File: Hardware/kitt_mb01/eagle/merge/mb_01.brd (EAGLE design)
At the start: 160 x 100 mm, 123 parts, among them CON1 ARDUINO_UNO, IC1.01 RT8293A, IC2.00 BQ24266RGET, IC3.01 LSM9DS1, P2 S2B-PH-K-S(LF)(SN), U6.01 TPS61032RSARPSDO-G16, U7.01 SI1922EDH, X7.02 HEAD-LIGHT, X7.03 TAIL-LIGHT, X7.05 MOTOR

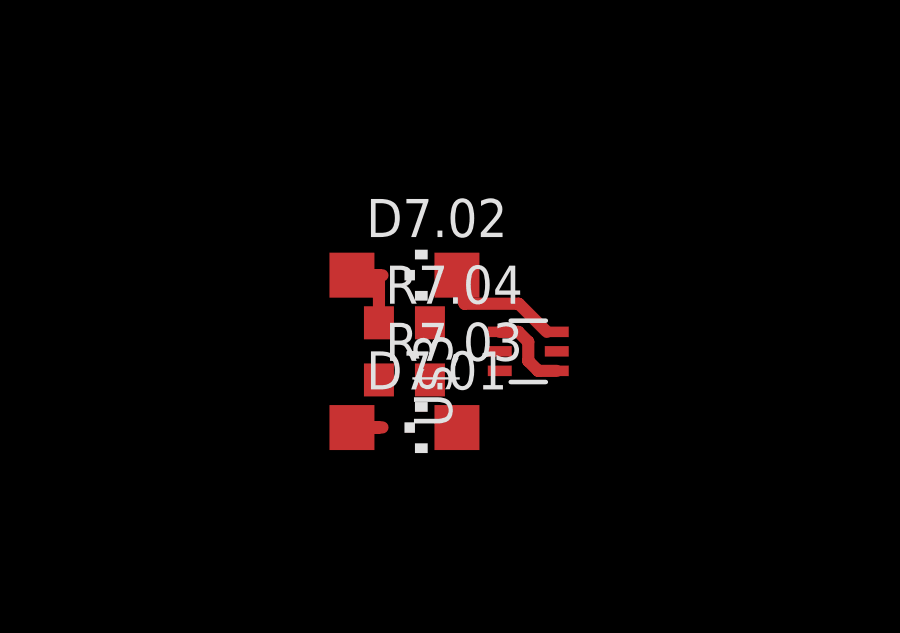
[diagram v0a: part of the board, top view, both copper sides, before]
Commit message: snapshot of board merge
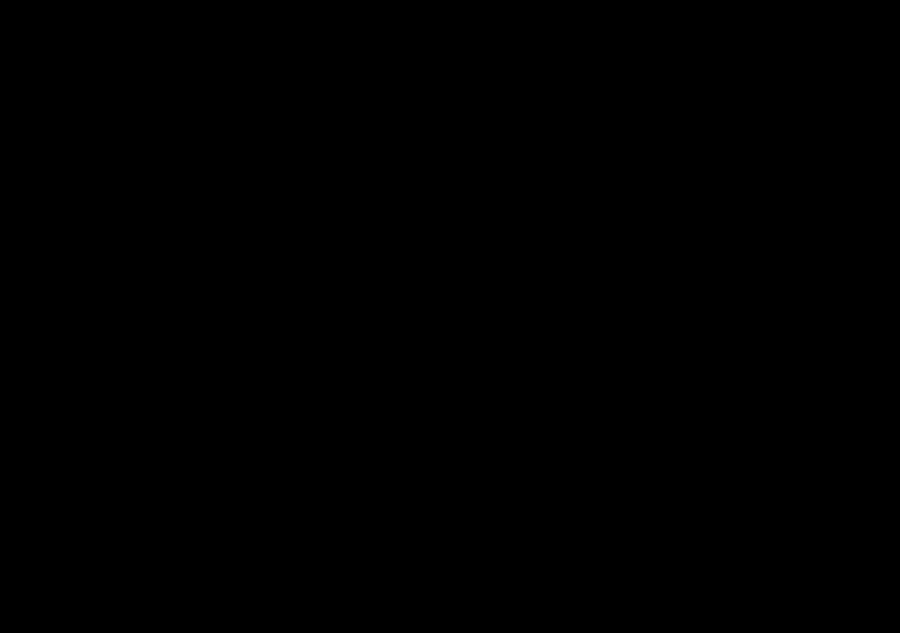
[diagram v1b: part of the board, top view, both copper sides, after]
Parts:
- removed D7.01, D7.02: (no value), led:CHIPLED_1206
- removed R7,03, R7.04: 330R, rcl:R0603
- U$3: value SI1922EDH -> (none); device kitt.ic:SC70-6 -> frames:A4L-LOC
- moved U$3 110.4 mm to (-48.3, -42.5), turned to 0 degrees
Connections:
- removed net N$3: D7.01.C, U$3.6
- removed net N$4: D7.01.A, R7,03.1
- removed net N$5: D7.02.A, R7.04.1
- removed net N$7: D7.02.C, U$3.3
- net +3V3: no longer R7,03.2, R7.04.2
- net GND: no longer U$3.1, U$3.4
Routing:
- net N$7: track 4.12 -> 0.00 mm
- net N$5: track 3.51 -> 0.00 mm
- net GND: track 245.3 -> 242.5 mm
- net N$4: track 1.92 -> 0.00 mm
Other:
- board text added: "D.Hoeginger/A.Gessler"
- board text added: "KITT-MB01 PCB LAYOUT"
- board text added: "Kit for Intelligent and Trainable Trackcars"
- board text removed: "<-- IDK"
- board text removed: "GND@2"
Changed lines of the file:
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@@
 <layers>
 <layer number="1" name="Top" color="4" fill="1" visible="yes" active="yes"/>
-<layer number="2" name="Route2" color="29" fill="0" visible="no" active="yes"/>
+<layer number="2" name="Route2" color="29" fill="0" visible="yes" active="yes"/>
 <layer number="3" name="Route3" color="24" fill="9" visible="yes" active="yes"/>
 <layer number="14" name="Route14" color="1" fill="6" visible="no" active="no"/>
@@
 <wire x1="102.6" y1="73.9" x2="49.1" y2="73.9" width="0.4064" layer="20"/>
 <wire x1="46.7" y1="71.4" x2="46.7" y2="23.1" width="0.4064" layer="20"/>
-<text x="20.16125" y="7.77875" size="1.778" layer="2">GND@2</text>
-<text x="147.32" y="4.60375" size="1.778" layer="2">GND@2</text>
-<text x="143.03375" y="87.78875" size="1.778" layer="2">GND@2</text>
-<text x="8.5725" y="89.8525" size="1.778" layer="2">GND@2</text>
 <text x="48.26" y="64.92875" size="1.9304" layer="25" font="vector">+</text>
 <text x="102.5525" y="35.40125" size="1.016" layer="25" font="vector" rot="R90">SHUNT</text>
@@
 <text x="106.600625" y="46.51375" size="1.778" layer="51">&lt;-- Head Light</text>
 <hole x="101.6" y="27.94" drill="1.6"/>
-<text x="15.5575" y="52.07" size="1.6764" layer="49" rot="R90">&lt;-- IDK</text>
 <text x="20.32" y="37.7825" size="1.6764" layer="49">SPEEDBOARD --&gt;
 LAPDETECTOR --&gt;</text>
@@
 <text x="91.7575" y="8.5725" size="1.778" layer="48">RAILS POURS</text>
 <text x="70.1675" y="6.0325" size="1.778" layer="48">ARDUINO&lt;-&gt;RAILS</text>
+<text x="168.91" y="-22.225" size="1.9304" layer="48" font="vector">D.Hoeginger/A.Gessler</text>
+<text x="114.3" y="-21.9075" size="1.9304" layer="48" font="vector">KITT-MB01 PCB LAYOUT</text>
+<text x="114.3" y="-36.5125" size="1.9304" layer="48" font="vector">Kit for Intelligent and
+Trainable Trackcars</text>
 </plain>
 <attributes>
@@
 <attribute name="MPN" value="" x="102.71125" y="46.51375" size="1.016" layer="27" font="vector" rot="R270" display="off"/>
 </element>
-<element name="D7.01" library="led" package="CHIPLED_1206" value="" x="14.049375" y="43.100625" rot="R270"/>
-<element name="U$3" library="kitt.ic" package="SC70-6" value="SI1922EDH" x="18.176875" y="45.640625" rot="R90"/>
-<element name="R7,03" library="rcl" package="R0603" value="330R" x="14.049375" y="44.688125"/>
-<element name="R7.04" library="rcl" package="R0603" value="330R" x="14.049375" y="46.593125"/>
-<element name="D7.02" library="led" package="CHIPLED_1206" value="" x="14.049375" y="48.180625" rot="R270"/>
 <element name="R0.02" library="rcl" package="R1206" value="SHUNT" x="51.7525" y="56.753125" rot="R270"/>
 <element name="D7.03" library="led" package="CHIPLED_1206" value="" x="101.6" y="54.61" rot="MR90"/>
@@
 <element name="REF1" library="kitt.refs" package="REF_LAYERS" value="REF.LAYERS" x="102.5525" y="67.945" rot="R270"/>
 <element name="REF2" library="kitt.refs" package="REF_LOGO_UASUA" value="REF.LOGO.UASUA" x="77.63" y="65.405" rot="MR270"/>
+<element name="U$3" library="frames" package="A4L-LOC" value="" x="-48.26" y="-42.545"/>
 </elements>
 <signals>
@@
 <wire x1="92.948125" y1="40.9575" x2="94.853125" y2="39.0525" width="1.6764" layer="1"/>
 <wire x1="94.853125" y1="39.0525" x2="100.0125" y2="39.0525" width="1.6764" layer="1"/>
-<contactref element="U$3" pad="1"/>
-<contactref element="U$3" pad="4"/>
-<wire x1="17.226875" y1="46.290625" x2="17.844375" y2="46.290625" width="0.4064" layer="1"/>
-<wire x1="17.844375" y1="46.290625" x2="18.176875" y2="45.958125" width="0.4064" layer="1"/>
-<wire x1="18.176875" y1="45.958125" x2="18.176875" y2="45.323125" width="0.4064" layer="1"/>
-<wire x1="18.176875" y1="45.323125" x2="18.509375" y2="44.990625" width="0.4064" layer="1"/>
-<wire x1="19.126875" y1="44.990625" x2="18.509375" y2="44.990625" width="0.4064" layer="1"/>
 <wire x1="69.8025" y1="41.91" x2="67.945" y2="41.91" width="0.4064" layer="1"/>
 <wire x1="67.945" y1="41.91" x2="66.28" y2="41.91" width="0.4064" layer="1"/>
@@
 <wire x1="103.505" y1="27.785" x2="103.35" y2="27.94" width="0.6096" layer="16"/>
 <wire x1="89.349375" y1="47.550625" x2="88.9" y2="47.3225" width="0" layer="19" extent="1-16"/>
-<wire x1="19.126875" y1="44.990625" x2="48.26" y2="55.331125" width="0" layer="19" extent="1-1"/>
 </signal>
 <signal name="+12V">
@@
 <wire x1="84.29625" y1="43.4975" x2="84.29625" y2="43.244375" width="0.254" layer="1"/>
 <wire x1="84.29625" y1="43.244375" x2="84.61375" y2="43.00625" width="0.254" layer="1"/>
-<contactref element="R7.04" pad="2"/>
-<contactref element="R7,03" pad="2"/>
 <contactref element="R7.01" pad="2"/>
 <contactref element="R7,01" pad="2"/>
@@
 <wire x1="51.865" y1="50.8" x2="54.9275" y2="50.8" width="1.016" layer="1"/>
 <wire x1="76.835" y1="42.148125" x2="77.94625" y2="42.148125" width="0" layer="19" extent="1-3"/>
-<wire x1="14.899375" y1="46.593125" x2="51.865" y2="50.8" width="0" layer="19" extent="1-1"/>
-<wire x1="14.899375" y1="44.688125" x2="14.899375" y2="46.593125" width="0" layer="19" extent="1-1"/>
 </signal>
 <signal name="N$17">
@@
 <wire x1="60.6275" y1="62.70625" x2="58.57875" y2="62.70875" width="0" layer="19" extent="1-1"/>
 </signal>
-<signal name="N$3">
-<contactref element="D7.01" pad="C"/>
-<contactref element="U$3" pad="6"/>
-<wire x1="15.539375" y1="43.100625" x2="15.799375" y2="43.100625" width="0.4064" layer="1"/>
-<wire x1="15.799375" y1="43.100625" x2="17.226875" y2="44.990625" width="0" layer="19" extent="1-1"/>
-</signal>
-<signal name="N$4">
-<contactref element="R7,03" pad="1"/>
-<contactref element="D7.01" pad="A"/>
-<wire x1="13.316875" y1="43.105625" x2="12.299375" y2="43.100625" width="0.4064" layer="1"/>
-<wire x1="13.199375" y1="43.100625" x2="12.299375" y2="43.100625" width="0.4064" layer="1"/>
-<wire x1="13.316875" y1="43.105625" x2="13.199375" y2="44.688125" width="0" layer="19" extent="1-1"/>
-</signal>
-<signal name="N$5">
-<contactref element="R7.04" pad="1"/>
-<contactref element="D7.02" pad="A"/>
-<wire x1="13.316875" y1="48.175625" x2="12.299375" y2="48.180625" width="0.4064" layer="1"/>
-<wire x1="13.199375" y1="46.593125" x2="13.199375" y2="48.180625" width="0.4064" layer="1"/>
-<wire x1="13.199375" y1="48.180625" x2="12.299375" y2="48.180625" width="0.4064" layer="1"/>
-</signal>
-<signal name="N$7">
-<contactref element="D7.02" pad="C"/>
-<contactref element="U$3" pad="3"/>
-<wire x1="18.796875" y1="46.290625" x2="17.859375" y2="47.228125" width="0.4064" layer="1"/>
-<wire x1="17.859375" y1="47.228125" x2="16.051875" y2="47.228125" width="0.4064" layer="1"/>
-<wire x1="16.051875" y1="47.228125" x2="15.799375" y2="48.180625" width="0.4064" layer="1"/>
-<wire x1="18.796875" y1="46.290625" x2="19.126875" y2="46.290625" width="0" layer="19" extent="1-1"/>
-</signal>
 <signal name="N$25">
